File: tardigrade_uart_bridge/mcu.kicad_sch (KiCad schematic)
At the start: 1 part, among them U1 ATmega328P-A

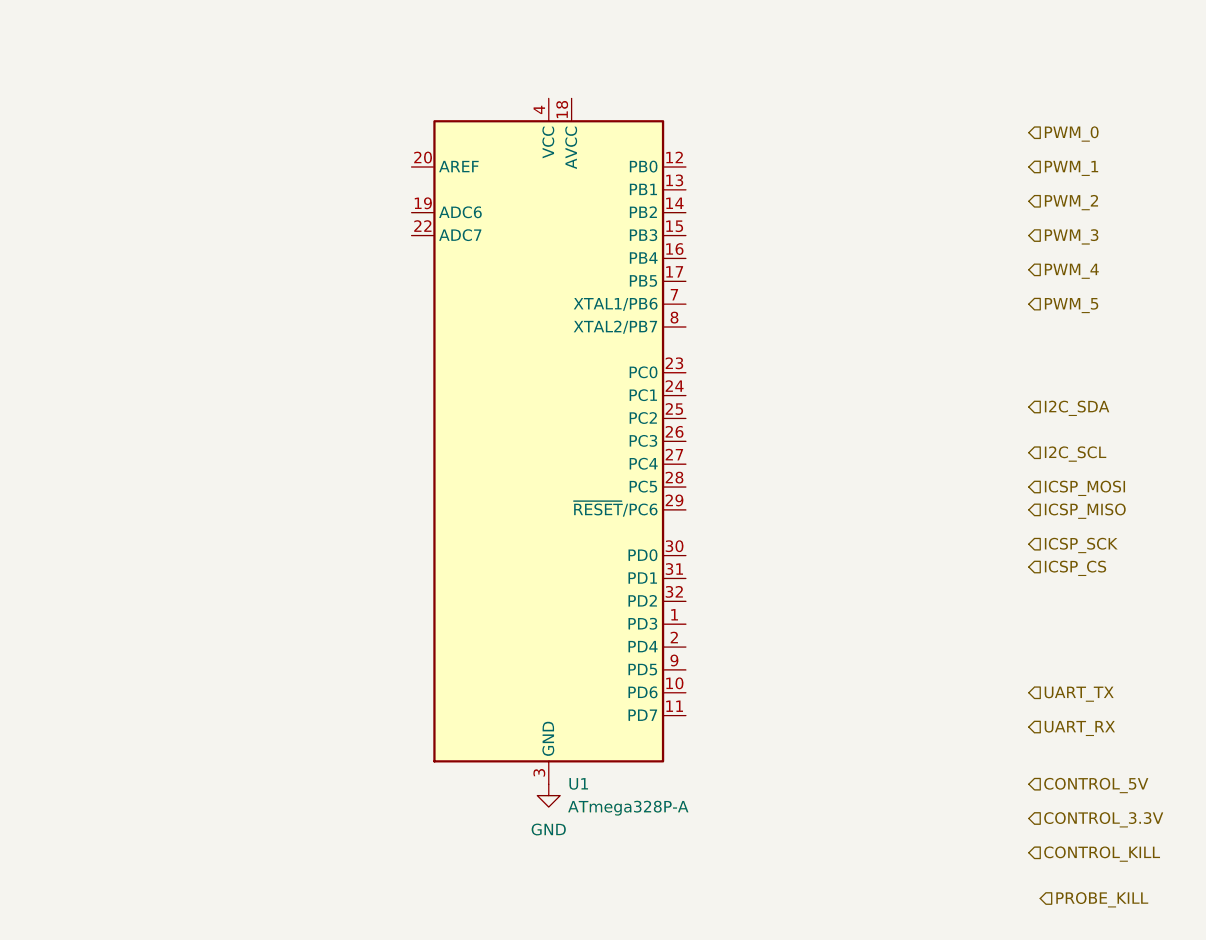
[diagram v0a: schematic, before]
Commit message: added basic passives for mcu
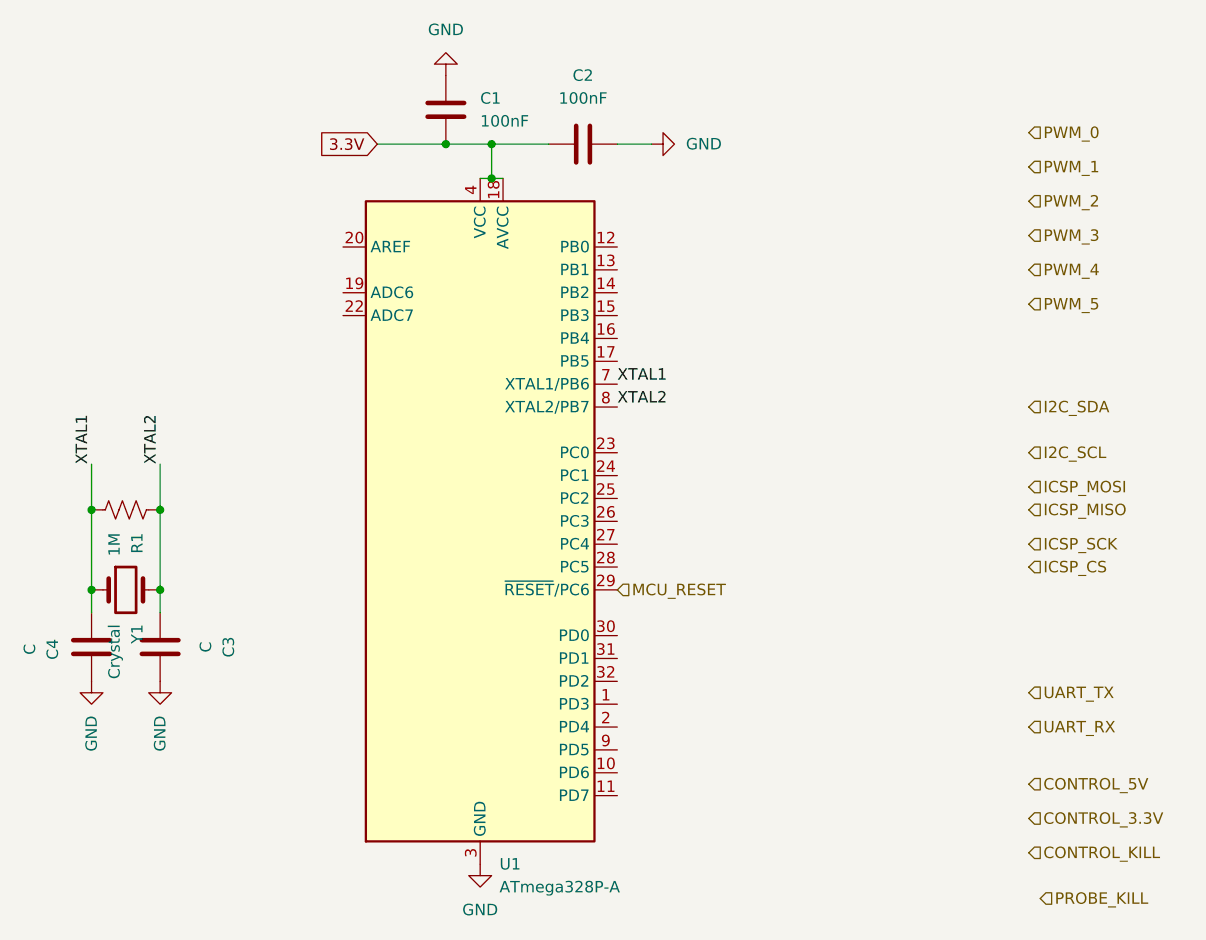
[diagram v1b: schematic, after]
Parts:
- added C1, C2: 100nF, symbol Device:C
- added C3, C4: C, symbol Device:C
- added R1: 1M, symbol Device:R_US
- added Y1: Crystal, symbol Device:Crystal
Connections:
- net GND: now also C1.1, C2.2, C3.2, C4.2
- net 3.3V: now reaches U1.18 (AVCC)
- net 3.3V: now also U1.4 (VCC), U1.6 (VCC), C1.2, C2.1
- net MCU_RESET: now reaches U1.29 (~{RESET}/PC6)
- net XTAL1: now reaches U1.7 (XTAL1/PB6)
- net XTAL1: now also C4.1, R1.1, Y1.1
- net XTAL2: now reaches U1.8 (XTAL2/PB7)
- net XTAL2: now also C3.1, R1.2, Y1.2
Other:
- moved on the sheet: U1
